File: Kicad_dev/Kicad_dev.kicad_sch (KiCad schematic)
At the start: 3 parts, among them Q1 IRF540N

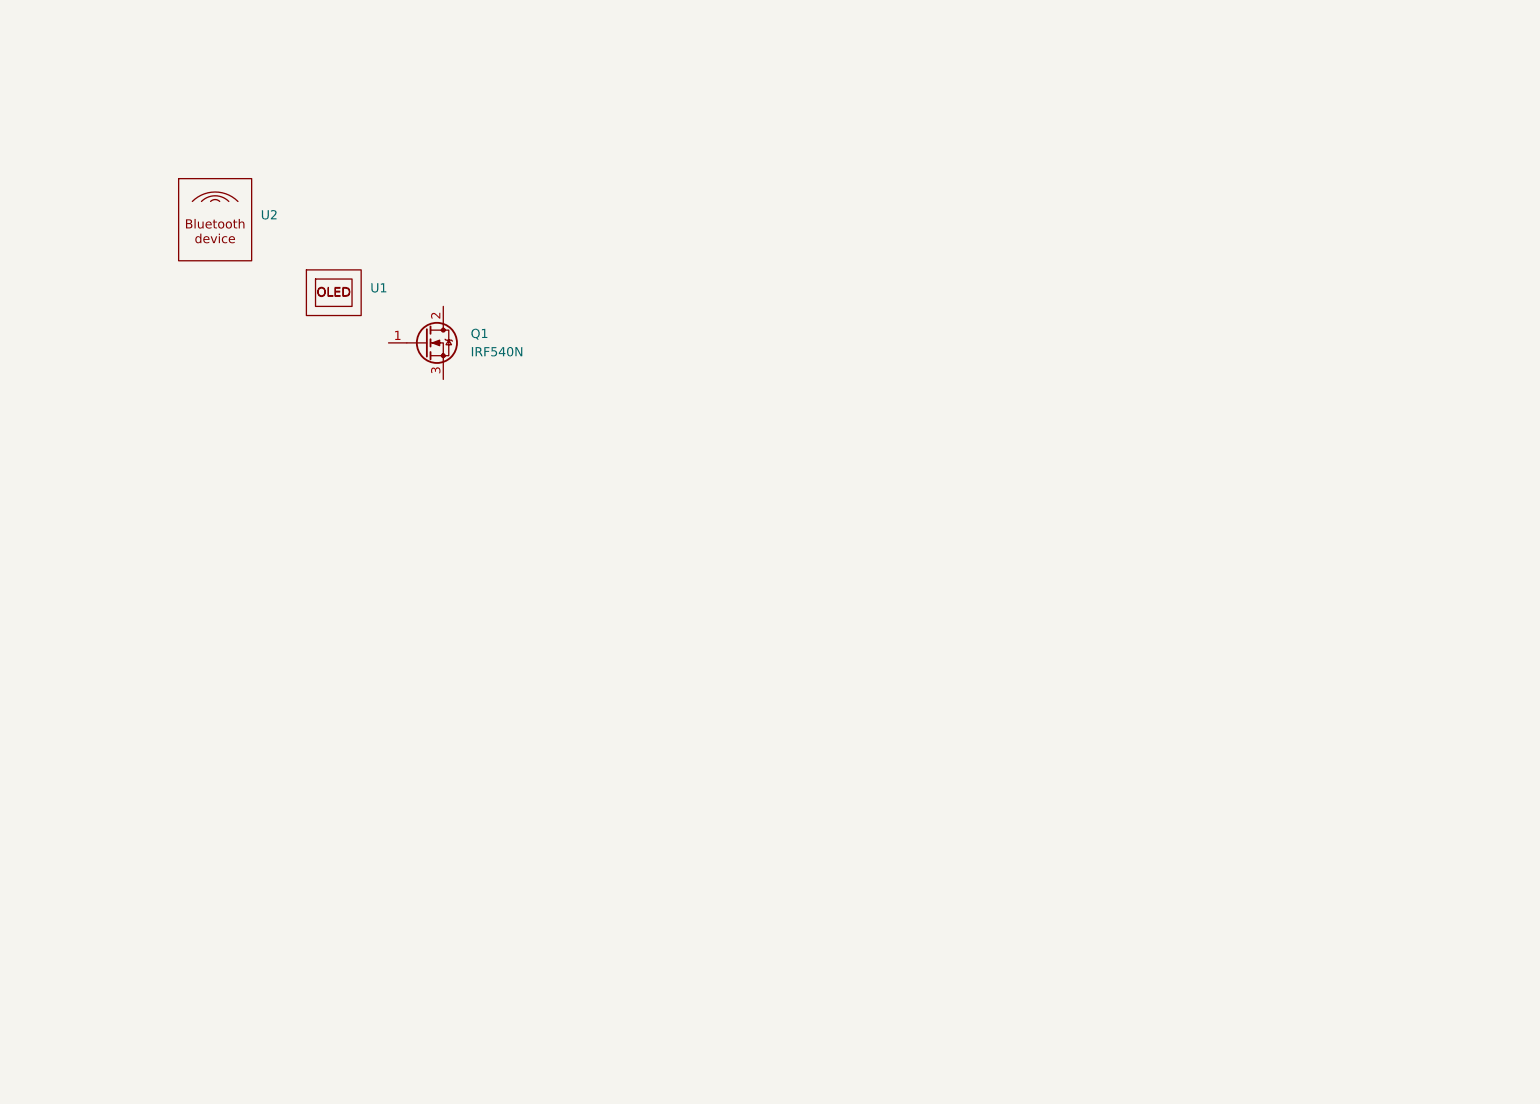
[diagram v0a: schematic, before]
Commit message: Add drawing file (attempting)
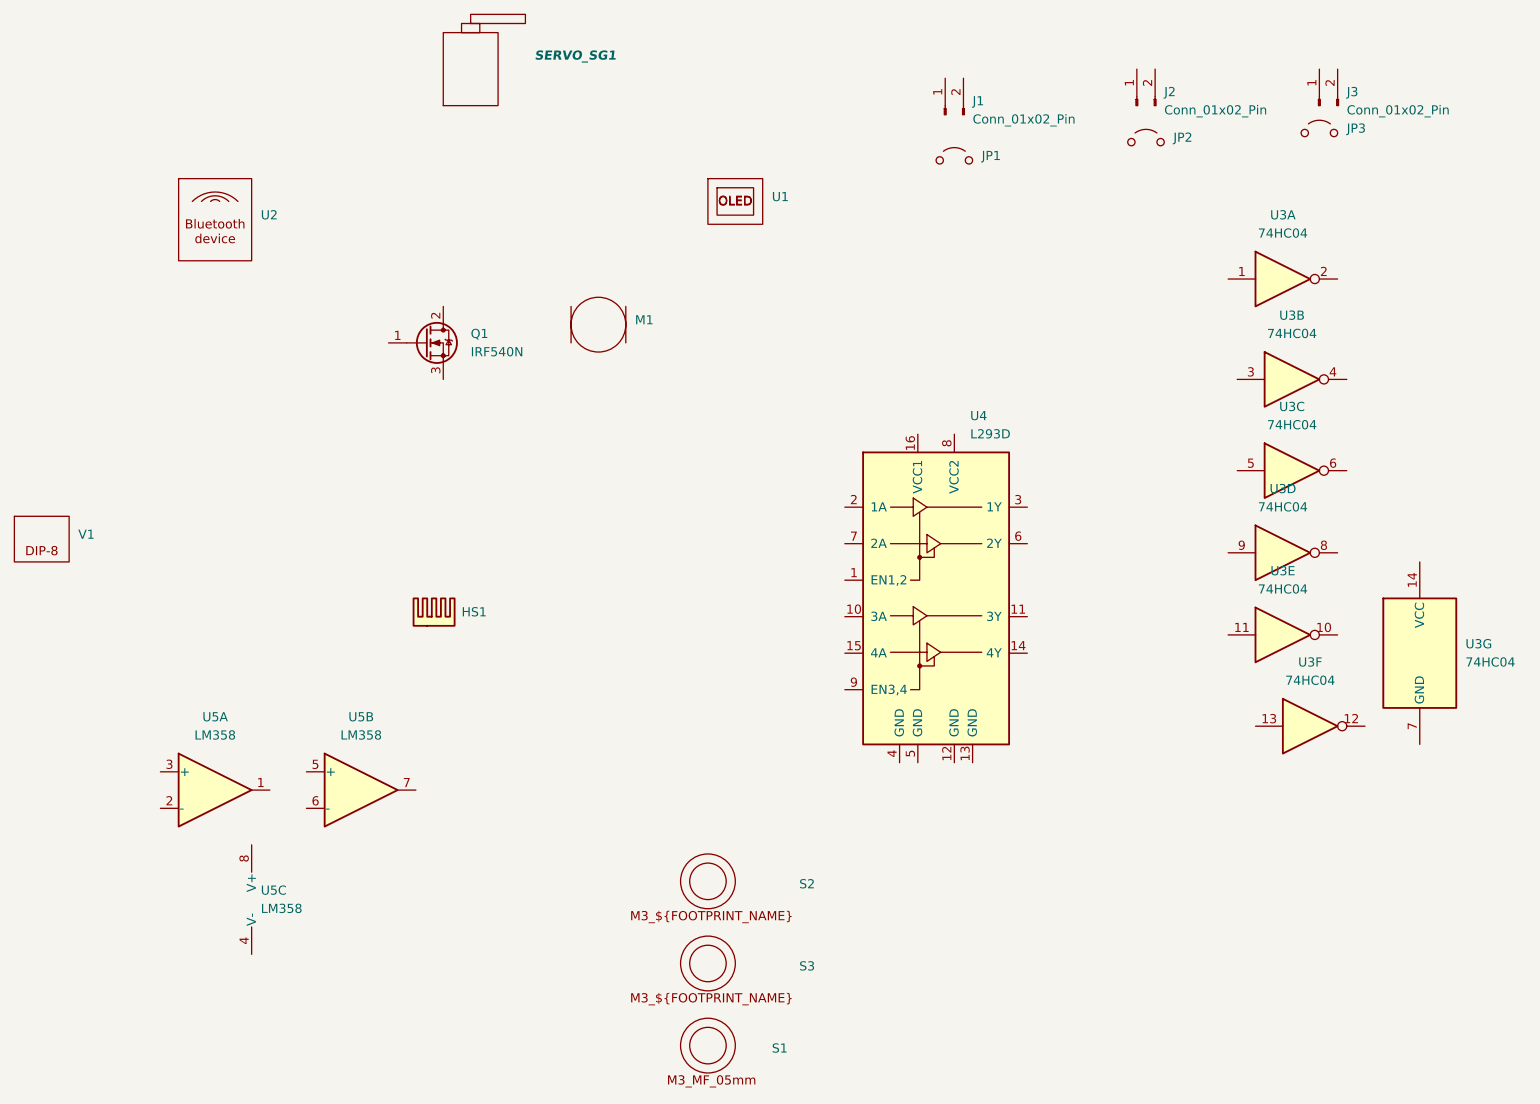
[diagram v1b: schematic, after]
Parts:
- removed U1: ~, symbol CREPP_Screens:OLED_SSD1306_0.96_inches_breakout
- added HS1: Heatsink [CREPP], CREPP_Heatsinks:HeastSink_MOSFET_15mm_10mm_20mm, symbol CREPP_Heatsinks:Heatsink
- added J1, J2, J3: Conn_01x02_Pin, Connector_PinHeader_2.54mm:PinHeader_1x02_P2.54mm_Vertical, symbol Connector:Conn_01x02_Pin
- added JP1: Jumper_2.54mm_black, CREPP_Jumpers:Jumper_2.54mm_black, symbol CREPP_Jumpers:Jumper_2.54mm_black
- added JP2: Jumper_2.54mm_red, CREPP_Jumpers:Jumper_2.54mm_red, symbol CREPP_Jumpers:Jumper_2.54mm_red
- added JP3: Jumper_2.54mm_blue, CREPP_Jumpers:Jumper_2.54mm_blue, symbol CREPP_Jumpers:Jumper_2.54mm_blue
- added M1: ~, symbol CREPP_Motors:Motor_3V_6V
- added S1: ~, CREPP_Spacers:Spacer_M3_MF_05mm, symbol CREPP_Spacers:Spacer_M3_05mm_MF
- added S2, S3: ~, CREPP_Spacers:Spacer_M3_MF_05mm, symbol CREPP_Spacers:Spacer_M3_Parametric
- added SERVO_SG1: ~, CREPP_Servo:SG90_Servo, symbol CREPP_Servomotors:Servomotor_SG90
- added U1: ~, CREPP_Screens:SSD1306_OLED_Display(128x64), symbol CREPP_Screens:OLED_SSD1306_0.96
- added U3: 74HC04, Package_DIP:DIP-14_W7.62mm_Socket, symbol CREPP_Logic:74HC04_THT
- added U4: L293D, Package_DIP:DIP-16_W7.62mm_Socket, symbol CREPP_Drivers_Motors:L293D_THT
- added U5: LM358, Package_DIP:DIP-8_W7.62mm_Socket, symbol CREPP_AOP_THT:LM358
- added V1: ~, CREPP_DIP:DIP-8_W7.62mm, symbol CREPP_DIP:DIP-8-Device
